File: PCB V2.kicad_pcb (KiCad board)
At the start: 2 copper layers, 17 parts, among them J1 Conector IR, J10 Conector ultrassonico esquerdo, J11 Conector ultrassonico central, J12 Conector ultrassonico direito, J13 Conector LED Extra, J14 Conector LORA, J15 ENCO_SW_Esq, J16 ENCO_SW_Dir, J18 LEDs, J2 Conector bluetooth, J3 Conector Acelerometro, J5 Conector servo, J7 Conector motor direito, J8 Conector motor esquerdo, J9 Conector alimentacao sensores

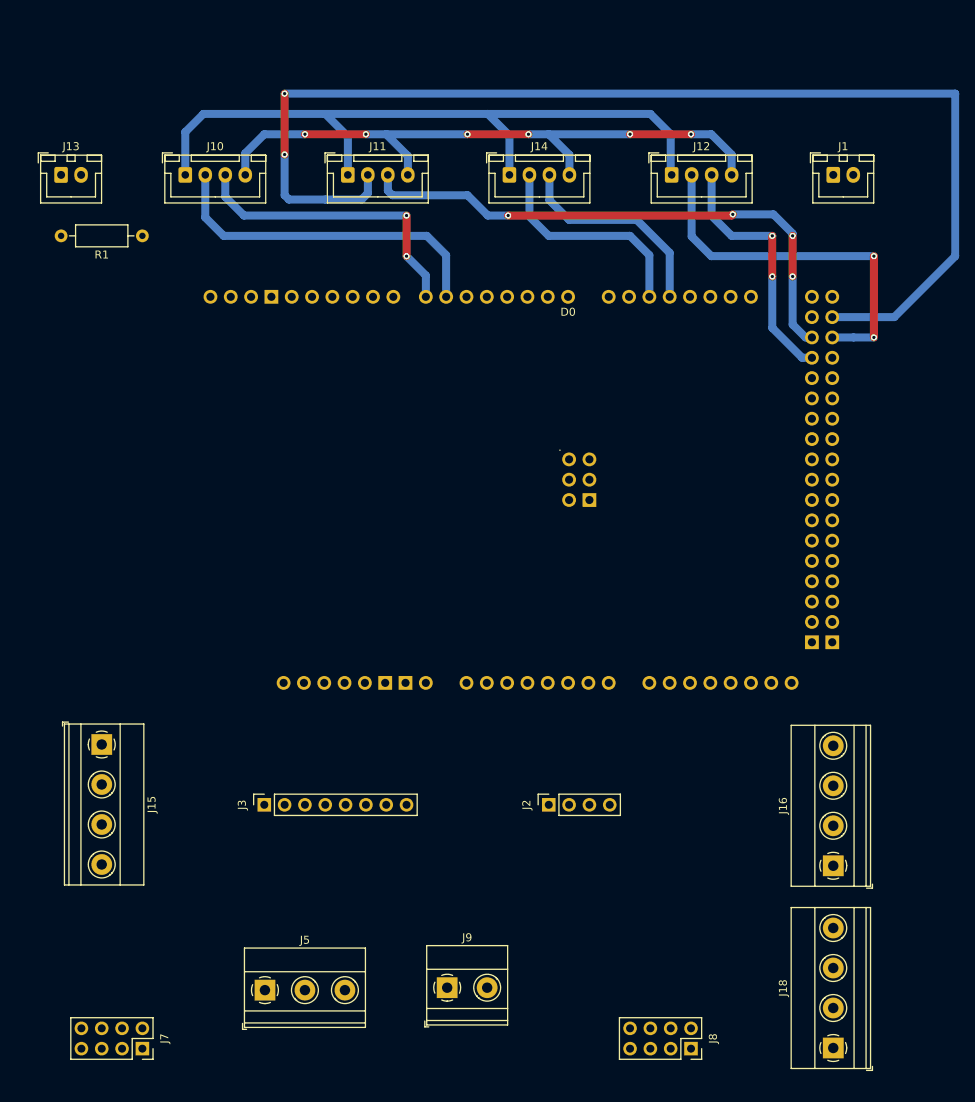
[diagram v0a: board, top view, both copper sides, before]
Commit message: feat: finalizacao da versao 2 da pcb
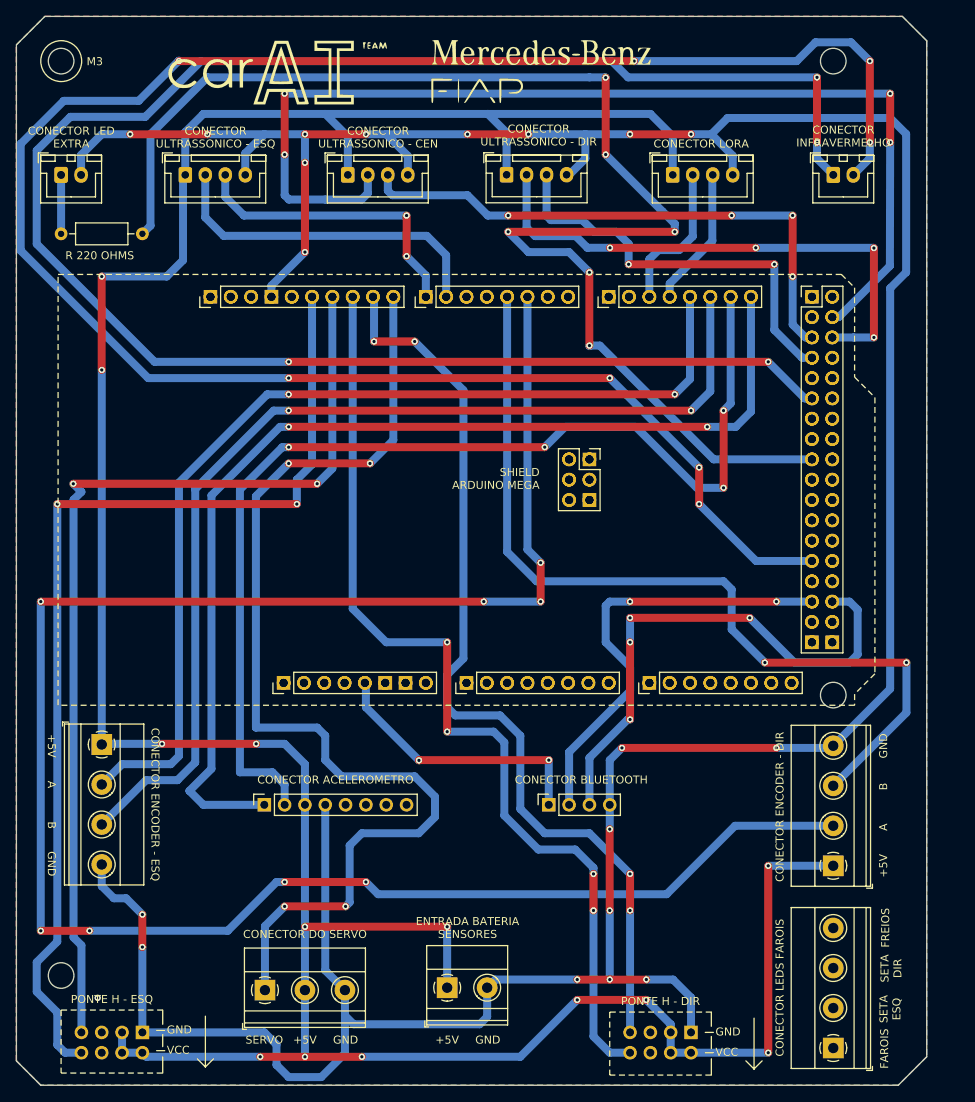
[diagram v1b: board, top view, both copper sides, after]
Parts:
- added G***: LOGO, LOGO, F.Cu at (142.1, 37.9)
- added REF**: PinHeader_1x08_P2.54mm_Vertical, Connector_PinHeader_2.54mm:PinHeader_1x08_P2.54mm_Vertical, F.Cu at (157.4, 66.0)
- added REF**: MountingHole_3.2mm_M3, MountingHole:MountingHole_3.2mm_M3, F.Cu at (185.4, 36.6)
- added REF**: MountingHole_3.2mm_M3, MountingHole:MountingHole_3.2mm_M3, F.Cu at (185.4, 115.8)
- added REF**: PinHeader_1x08_P2.54mm_Vertical, Connector_PinHeader_2.54mm:PinHeader_1x08_P2.54mm_Vertical, F.Cu at (116.7, 114.3)
- added REF**: PinSocket_2x03_P2.54mm_Vertical, Connector_PinSocket_2.54mm:PinSocket_2x03_P2.54mm_Vertical, F.Cu at (154.9, 86.4)
- added REF**: PinHeader_1x08_P2.54mm_Vertical, Connector_PinHeader_2.54mm:PinHeader_1x08_P2.54mm_Vertical, F.Cu at (162.4, 114.3)
- added REF**: PinHeader_1x08_P2.54mm_Vertical, Connector_PinHeader_2.54mm:PinHeader_1x08_P2.54mm_Vertical, F.Cu at (134.5, 66.0)
- added REF**: MountingHole_3.2mm_M3, MountingHole:MountingHole_3.2mm_M3, F.Cu at (88.9, 36.6)
- added REF**: MountingHole_3.2mm_M3, MountingHole:MountingHole_3.2mm_M3, F.Cu at (88.9, 150.9)
- added REF**: PinHeader_1x10_P2.54mm_Vertical, Connector_PinHeader_2.54mm:PinHeader_1x10_P2.54mm_Vertical, F.Cu at (107.6, 66.0)
- added REF**: PinHeader_2x18_P2.54mm_Vertical, Connector_PinHeader_2.54mm:PinHeader_2x18_P2.54mm_Vertical, F.Cu at (182.8, 66.0)
- added REF**: PinHeader_1x08_P2.54mm_Vertical, Connector_PinHeader_2.54mm:PinHeader_1x08_P2.54mm_Vertical, F.Cu at (139.6, 114.3)
- J7, J8: moved to B.Cu
- moved J12 20.6 mm to (144.6, 50.8)
- moved J14 20.4 mm to (165.4, 50.8)
- moved R1 10.2 mm to (88.9, 58.2), turned to 0 degrees
- moved J7 2.03 mm to (99.1, 158.0), turned to 90 degrees
- moved J8 2.03 mm to (167.6, 158.0), turned to 90 degrees
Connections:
- J7 pad 1: 5V_Sen -> Earth
- J7 pad 2: Earth -> 5V_Sen
- J8 pad 1: 5V_Sen -> Earth
- J8 pad 2: Earth -> 5V_Sen
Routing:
- net Earth: track 80.4 -> 431.3 mm, vias 6 -> 19
- net 5V_Sen: track 90.7 -> 382.3 mm, vias 0 -> 14
- net IR2: track 0.00 -> 258.6 mm, vias 0 -> 8
- net ENCODER_Esq_1: track 0.00 -> 248.3 mm, vias 0 -> 8
- net IR1: track 0.00 -> 232.6 mm, vias 0 -> 4
- net LED_Extra: track 0.00 -> 172.0 mm, vias 0 -> 6
- net Servo: track 0.00 -> 136.3 mm, vias 0 -> 4
- net A_SDA: track 0.00 -> 135.2 mm, vias 0 -> 4
- net A_SCL: track 0.00 -> 134.3 mm, vias 0 -> 2
- net ENCODER_Dir_2: track 0.00 -> 130.3 mm, vias 0 -> 2
- net MD1: track 0.00 -> 129.8 mm, vias 0 -> 2
- net ENCODER_Dir_1: track 0.00 -> 124.8 mm, vias 0 -> 2
- net MD2: track 0.00 -> 124.5 mm, vias 0 -> 2
- net ME1: track 0.00 -> 120.9 mm, vias 0 -> 4
- net ME2: track 0.00 -> 116.5 mm, vias 0 -> 4
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- added copper zone on B.Cu, net Earth
- added copper zone on F.Cu, net Earth
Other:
- board outline added: 113.8 x 133.6 mm
- board text added: "+5V"
- board text added: "A"
- board text added: "B"
- board text added: "CONECTOR ACELEROMETRO"
- board text added: "CONECTOR BLUETOOTH"
- board text added: "CONECTOR DO SERVO"
- board text added: "CONECTOR ENCODER - DIR"
- board text added: "CONECTOR ENCODER - ESQ"
- board text added: "CONECTOR INFRAVERMELHO"
- board text added: "CONECTOR LED EXTRA"
- board text added: "CONECTOR LEDS FAROIS"
- board text added: "CONECTOR LORA"
- board text added: "CONECTOR ULTRASSONICO - CEN"
- board text added: "CONECTOR ULTRASSONICO - DIR"
- board text added: "CONECTOR ULTRASSONICO - ESQ"
- board text added: "ENTRADA BATERIA SENSORES"
- board text added: "FAROIS"
- board text added: "FREIOS"
- board text added: "GND"
- board text added: "M3"
- board text added: "PONTE H - DIR"
- board text added: "PONTE H - ESQ"
- board text added: "R 220 OHMS"
- board text added: "SERVO"
- board text added: "SETA DIR"
- board text added: "SETA ESQ"
- board text added: "SHIELD ARDUINO MEGA"
- board text added: "VCC"
